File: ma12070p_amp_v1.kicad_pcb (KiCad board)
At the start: 2 copper layers, 81 parts, among them J2 Screw_Terminal_01x04, J3 Screw_Terminal_01x02, U1 MA12070P, U2 TPS62175DQC

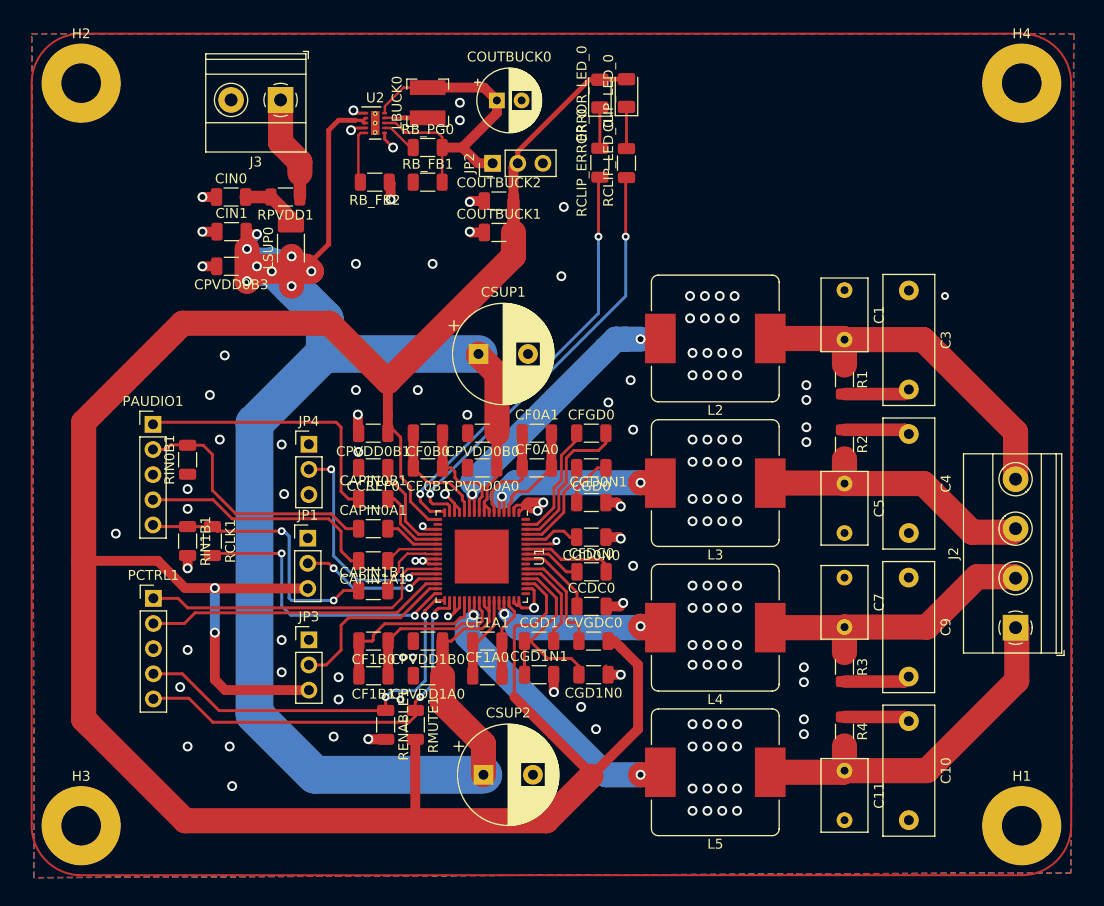
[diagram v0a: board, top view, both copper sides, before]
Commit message: small updates to pcb
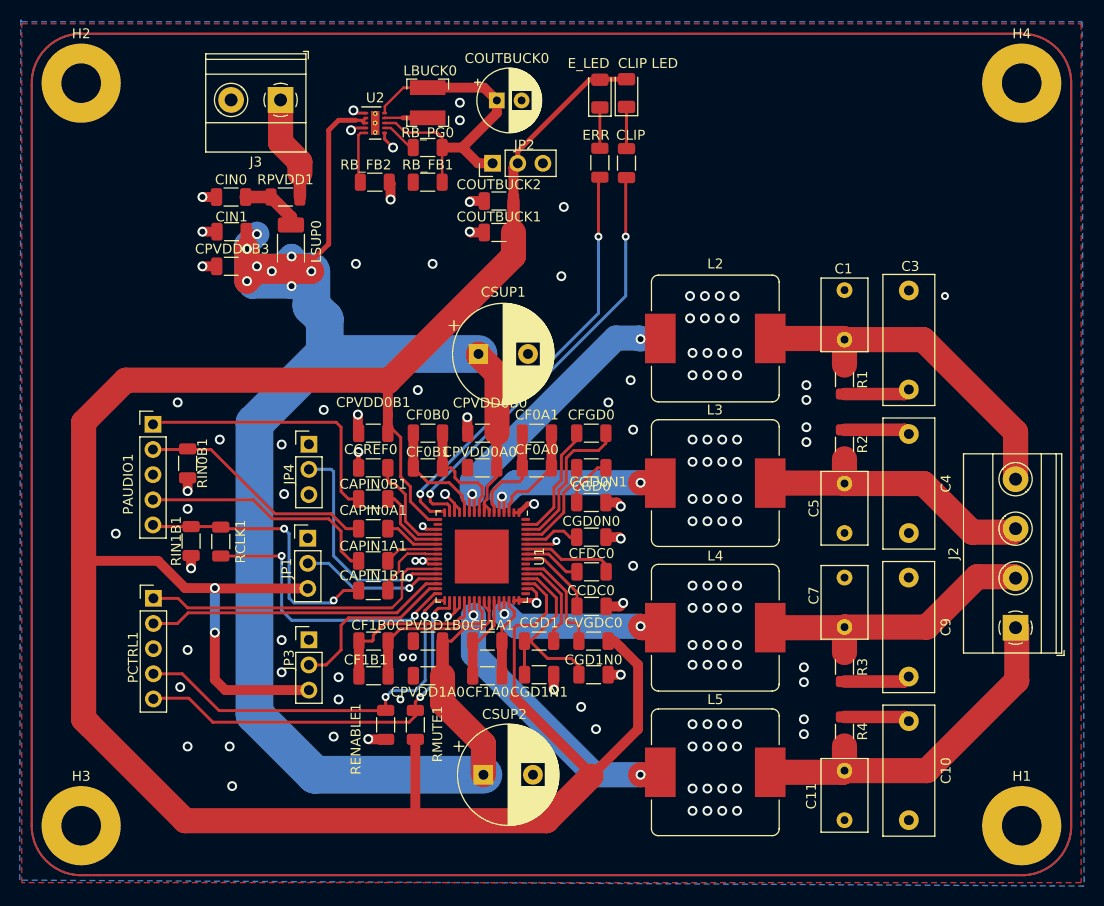
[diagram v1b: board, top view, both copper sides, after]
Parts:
- CLIP LED: renamed from CLIP_LED_0
- moved RCLK1 0.85 mm to (129.1, 96.3)
- moved RIN0B1 0.36 mm to (125.8, 88.4)
- moved RIN1B1 0.35 mm to (126.1, 96.2)
- renumbered RCLIP_LED_0 to CLIP, RCLIP_ERROR_0 to ERR, ERROR_LED_0 to E_LED
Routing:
- net /VDD: track 318.8 -> 314.0 mm
- net /PVDD: track 199.9 -> 195.7 mm
- net GND: track 57.2 -> 54.3 mm, vias 136 -> 134
- net Net-(CAPIN0A1-Pad1): track 26.6 -> 24.1 mm
- net AD1: track 13.8 -> 14.6 mm, vias 2 -> 1
- net CLK: track 29.6 -> 29.1 mm
- net AD0: vias 2 -> 1
